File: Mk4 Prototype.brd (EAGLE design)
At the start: 121.6 x 80 mm, 211 parts, among them IC1 MSP432E401, IC10 TPD3E001DRL, IC11 LMV358ID, IC12 SN74HC4066D, IC2 AS4C8M16SA-7TCN, IC3 CC3120MOD, IC4 MCP23017ML, IC5 SIM800C, IC6 SST26VF064B-104I/SM, IC7 TPD3E001DRL, IC8 BQ25601, IC9 TPS62082, J1 78723-1001, J2 ER-CON50HT-1, J3 2x5 1.27mm (NP), J4 GSM-COIL-ANT, Q1 2N7002PW, Q2 2N7002PW, Q3 CSD25402Q3A, Q8 CSD13202Q2, SW1 JOYSTICK, U2 ER-TFT024-3 (NP), U4 MIC-1X02, U5 LDMS1540S-01-R8-0.8-R, X1 FC-135R 32.768KHZ 9PF, X2 NX3225GA-25.000M-STD-CRG-2

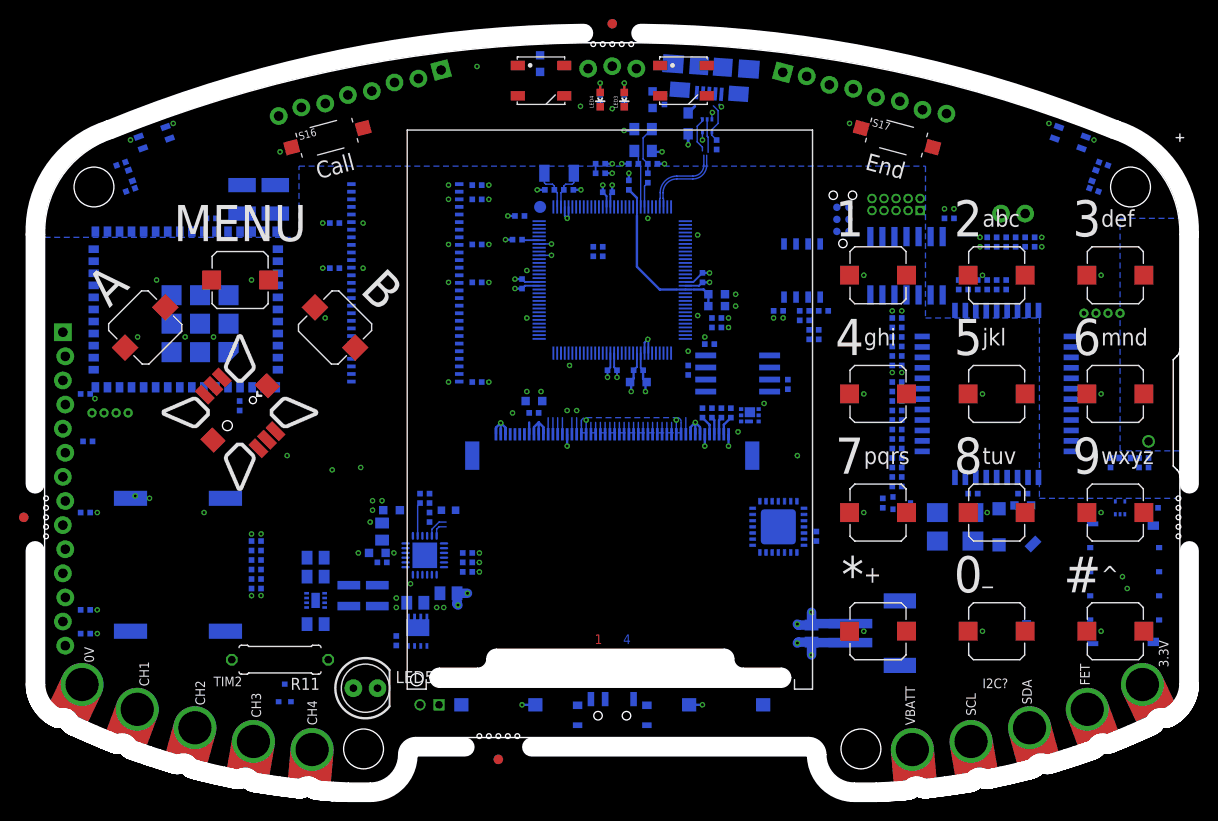
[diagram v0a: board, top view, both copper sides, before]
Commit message: Schematic should now have all the parts
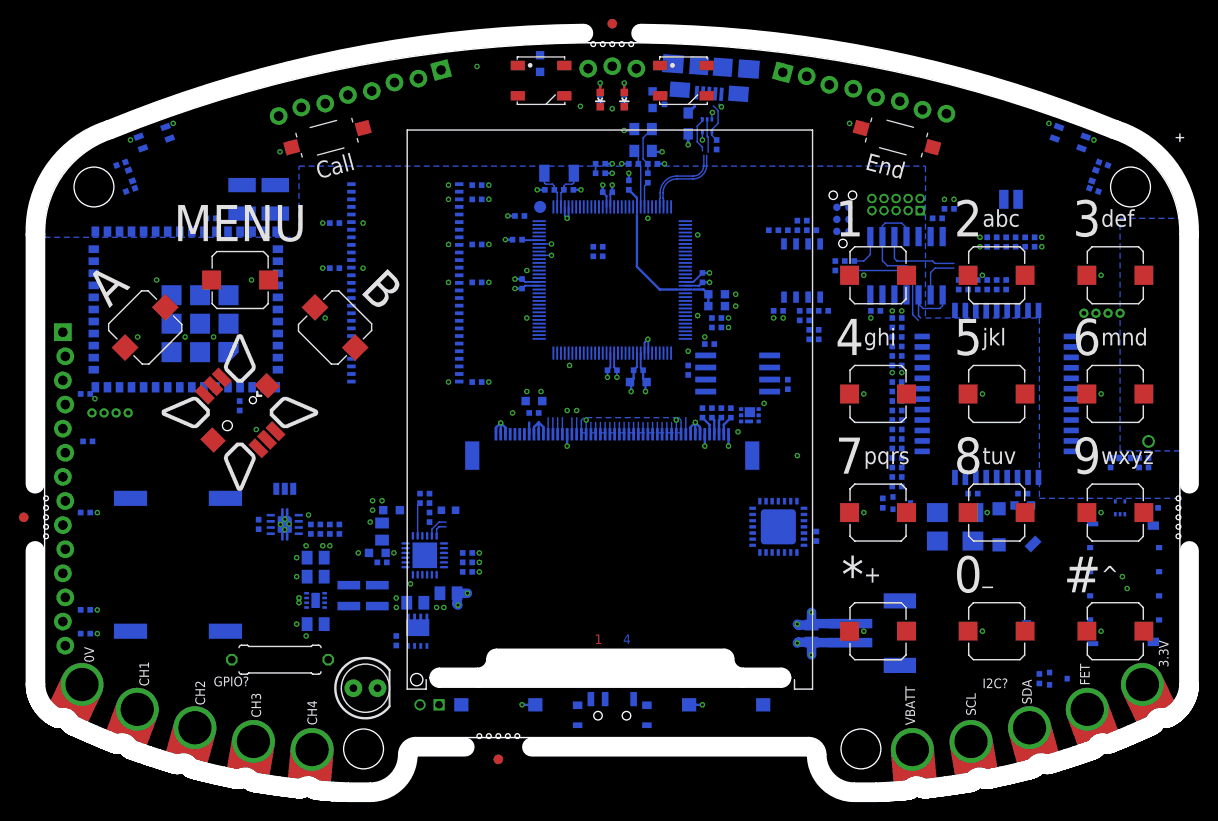
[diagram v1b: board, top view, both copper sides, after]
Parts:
- removed C59, C62, C63: 0402/10p/50V/X5R, TiLDA Mk4 Parts:C0402-SMALLER
- removed C60, C61: 0402/33p/50V/X5R, TiLDA Mk4 Parts:C0402-SMALLER
- added C78: 0402/1n/10V/X5R, TiLDA Mk4 Parts:C0402-SMALLER
- added C79: 0402/2n2/10V/X5R, TiLDA Mk4 Parts:C0402-SMALLER
- added C80, C81: 0402/100n/10V/X5R, TiLDA Mk4 Parts:C0402-SMALLER
- added C82, C83: 0402/220n/6V/X5R, TiLDA Mk4 Parts:C0402-SMALLER
- added IC13: TPA2066D1, TiLDA Mk4 Parts:VSON-8
- added R52: 0402/14K7/5%, TiLDA Mk4 Parts:R0402-SMALLER
- added R53: 0402/7K87/5%, TiLDA Mk4 Parts:R0402-SMALLER
- added R54, R55, R56: 0402/10K/5%, TiLDA Mk4 Parts:R0402-SMALLER
- added R57, R58: 0402/150K/1%, TiLDA Mk4 Parts:R0402-SMALLER
- added R59: 0402/10k/5%, TiLDA Mk4 Parts:R0402-SMALLER
- added SJ1: (no value), TiLDA Mk4 Parts:SJ_3
- C58: value 0402/33p/50V/X5R -> 0402/100n/10V/X5R
- U4: value MIC-1X02 -> MIC-4MM; device TiLDA Mk4 Parts:1X02 -> TiLDA Mk4 Parts:MIC-SMD-4MM
- moved Q2 81.5 mm to (47.0, 11.0), turned to 90 degrees
- moved C58 4.26 mm to (-37.2, 27.2)
- moved U4 2.12 mm to (42.0, 61.5)
- moved C71 1.00 mm to (35.5, 60.5)
- turned C47 to 0 degrees
- turned C65 to 90 degrees
- turned C67 to 90 degrees
- turned U5 to 90 degrees
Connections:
- new net MIC_MUX_N: IC12.11, IC12.9, IC5.10
- new net MIC_MUX_P: IC12.1, IC12.3, IC5.9
- new net MIC_PWM: R53.2
- new net MIC_PWM_AMP: C79.1, C80.2, C81.2, IC11.1, IC11.2
- new net MIC_PWM_N: C80.1, IC12.8, R54.1
- new net MIC_PWM_P: C81.1, IC12.4, R54.2
- new net MUX_A: IC12.12, IC12.13, R56.1
- new net MUX_B: IC12.5, IC12.6, R55.2
- new net N$10: IC13.4, R58.2
- new net N$11: IC13.3, R57.2
- new net N$12: C83.1, R57.1
- new net N$15: C82.1, R58.1
- new net N$2: C78.2, IC11.3, R52.2
- new net N$7: C79.2, R52.1, R53.1
- new net N$9: C58.1, IC13.1, IC13.6, SJ1.2
- new net SPK_AMP_N: IC13.8, U5.-
- new net SPK_AMP_P: IC13.5, U5.+
- net 3V3: now also R56.2
- net FET: now also R59.1
- net GND: now also C58.2, C78.1, IC13.7, IC13.PAD, R55.1, R59.2; no longer C59.2, C60.2, C61.2, C63.2
- net MIC_N: now also IC12.10, U4.-; no longer IC5.10, U4.2
- net MIC_P: now also IC12.2, U4.+; no longer IC5.9, U4.1
- net SPK_N: now also C82.2; no longer C58.2, C59.1, C61.1, C62.2, U5.-
- net SPK_P: now also C83.2; no longer C58.1, C60.1, C62.1, C63.1, U5.+
- net VBATT: now also C1.1, JP2.2, LED1.1, LED2.1
- net V_UNREG: no longer C1.1, JP2.2, LED1.1, LED2.1
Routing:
- net MIC_MUX_N: track 0.00 -> 16.6 mm
- net MIC_N: track 0.00 -> 8.79 mm
- net MIC_PWM_P: track 0.00 -> 7.78 mm
- net MIC_MUX_P: track 0.00 -> 7.45 mm
- net MIC_P: track 0.00 -> 5.01 mm
- net MIC_PWM_N: track 0.00 -> 3.86 mm
- net GND: vias 102 -> 106
- net 3V3: vias 37 -> 39
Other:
- outline, holes or cut-outs redrawn
- board text removed: "TIM2"
